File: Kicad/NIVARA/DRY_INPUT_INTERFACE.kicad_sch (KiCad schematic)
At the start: 6 parts, among them U4 LTV-357TB

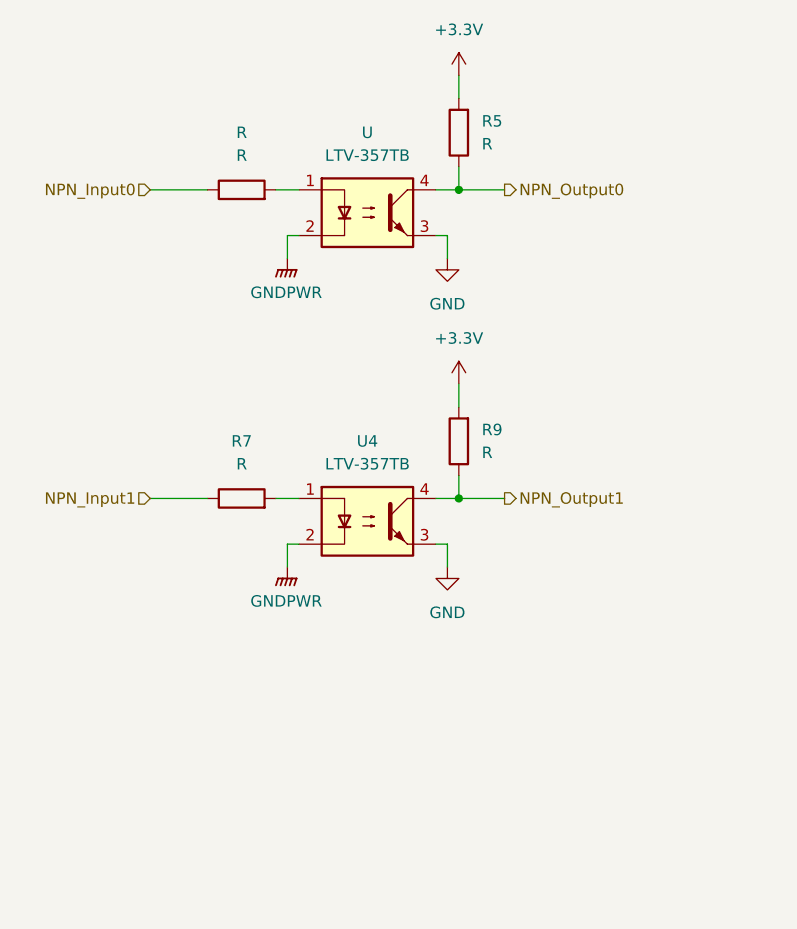
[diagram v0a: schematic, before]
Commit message: .
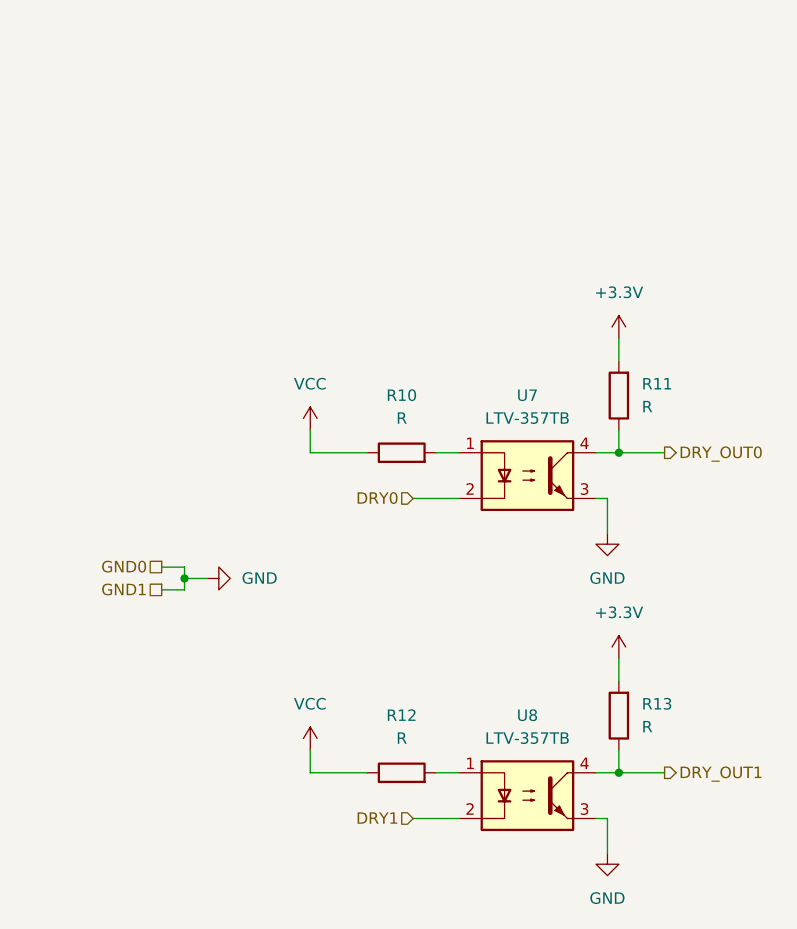
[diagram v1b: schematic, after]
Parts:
- removed R, R7: R, Resistor_SMD:R_0603_1608Metric, symbol Device:R
- removed R5, R9: R, symbol Device:R
- removed U, U4: LTV-357TB, Package_SO:SO-4_4.4x3.6mm_P2.54mm, symbol Isolator:LTV-357T
- added R10, R12: R, Resistor_SMD:R_0603_1608Metric, symbol Device:R
- added R11, R13: R, symbol Device:R
- added U7, U8: LTV-357TB, Package_SO:SO-4_4.4x3.6mm_P2.54mm, symbol Isolator:LTV-357T
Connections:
- net +3.3V: now also R11.2, R13.2
- net GND: now also U7.3, U8.3
- new net: R10.2, U7.1
- new net: R12.2, U8.1
- new net DRY0: U7.2
- new net DRY1: U8.2
- new net DRY_OUT0: R11.1, U7.4
- new net DRY_OUT1: R13.1, U8.4
- new net VCC: R10.1, R12.1
